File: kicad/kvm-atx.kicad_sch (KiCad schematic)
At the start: 18 parts, among them J1 ATX, J2 I2C0, J3 UART0, K1 AQW210EHA, K2 AQW210EHA, SW1 RESET, SW2 POWER

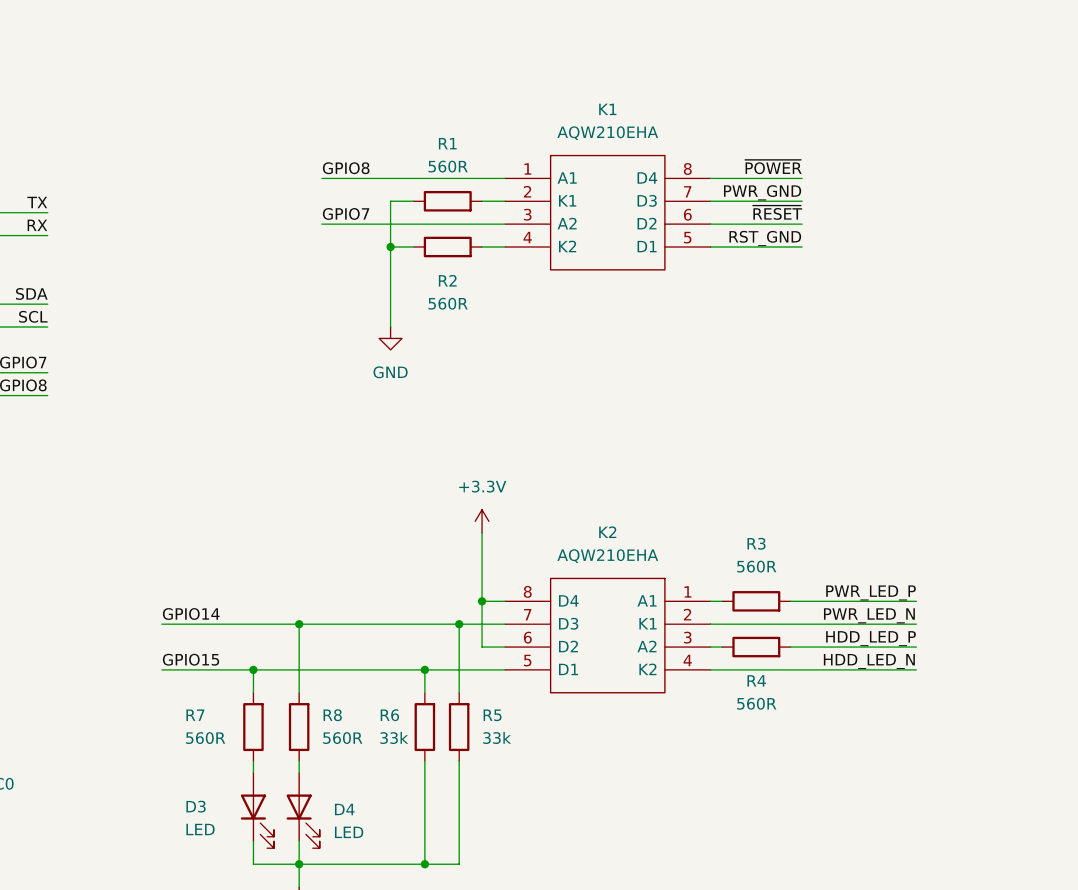
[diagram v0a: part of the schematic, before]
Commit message: WIP assembly version
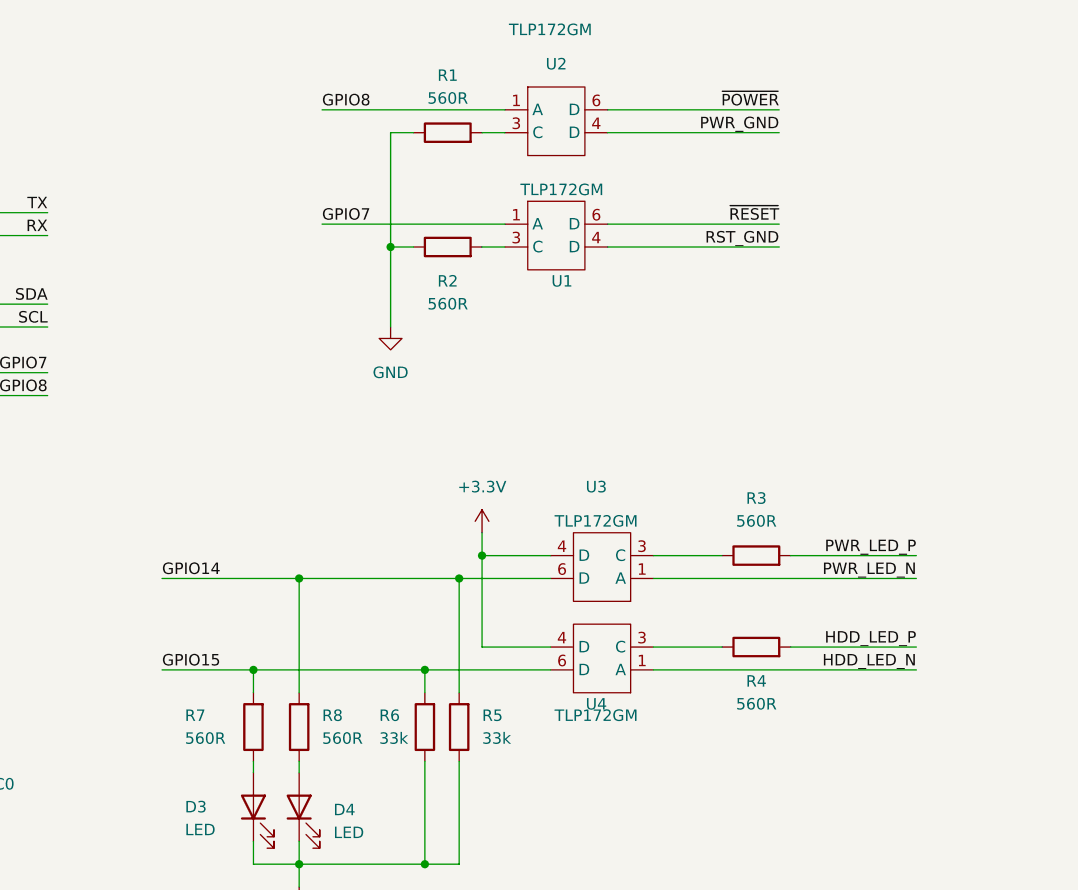
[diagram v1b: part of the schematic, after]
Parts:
- removed K1, K2: AQW210EHA, SOP254P962X315-8N, symbol 000:AQW210EHA
- added U1, U2, U3, U4: TLP172GM, 000:TLP172GM, symbol 000:TLP172GM
- D3, D4: footprint LED_SMD:LED_1206_3216Metric_Pad1.42x1.75mm_HandSolder -> LED_SMD:LED_0603_1608Metric
- R1, R2, R3, R4, R5, R6, R7, R8: footprint Resistor_SMD:R_1206_3216Metric_Pad1.30x1.75mm_HandSolder -> Resistor_SMD:R_0603_1608Metric
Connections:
- net +3.3V: now also U3.4 (D), U4.4 (D)
- net GPIO14: now also U3.6 (D)
- net GPIO15: now also U4.6 (D)
- net GPIO7: now also U1.1 (A)
- net GPIO8: now also U2.1 (A)
- net HDD_LED_N: now also U4.1 (A)
- net PWR_GND: now also U2.4 (D)
- net PWR_LED_N: now also U3.1 (A)
- net RST_GND: now also U1.4 (D)
- net ~{POWER}: now also U2.6 (D)
- net ~{RESET}: now also U1.6 (D)
- net at R3.1: now also U3.3 (C)
- net at R1.2: now also U2.3 (C)
- net at R2.2: now also U1.3 (C)
- net at R4.1: now also U4.3 (C)
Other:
- moved on the sheet: R1, R3
